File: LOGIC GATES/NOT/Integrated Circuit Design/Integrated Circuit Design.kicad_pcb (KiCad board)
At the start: 2 copper layers, 25 x 40 mm, 9 parts, among them J2 Conn_01x03_Socket, J3 Conn_01x03_Socket, Q1 QM6006D, Q3 QM6006D, U1 4011

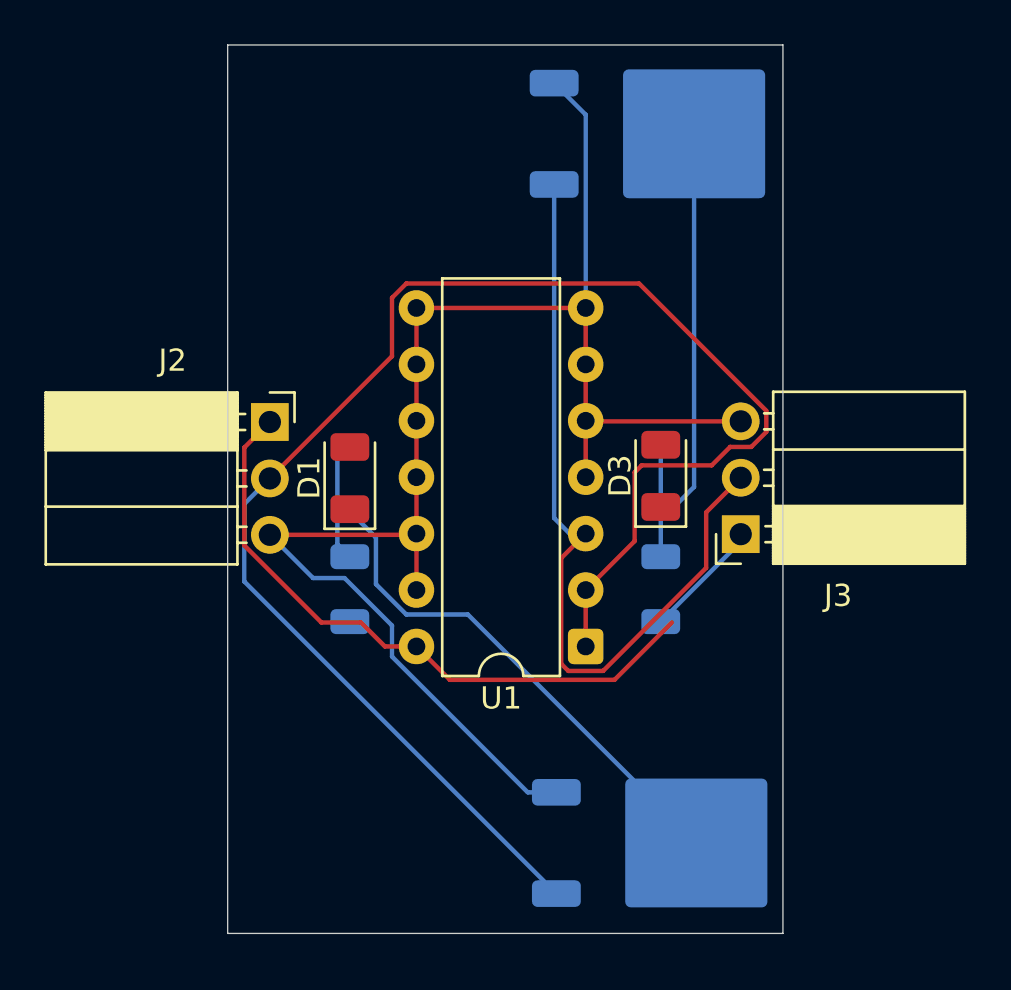
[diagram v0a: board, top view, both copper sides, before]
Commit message: Auto-update: 22.12.2025 16:16:21,18
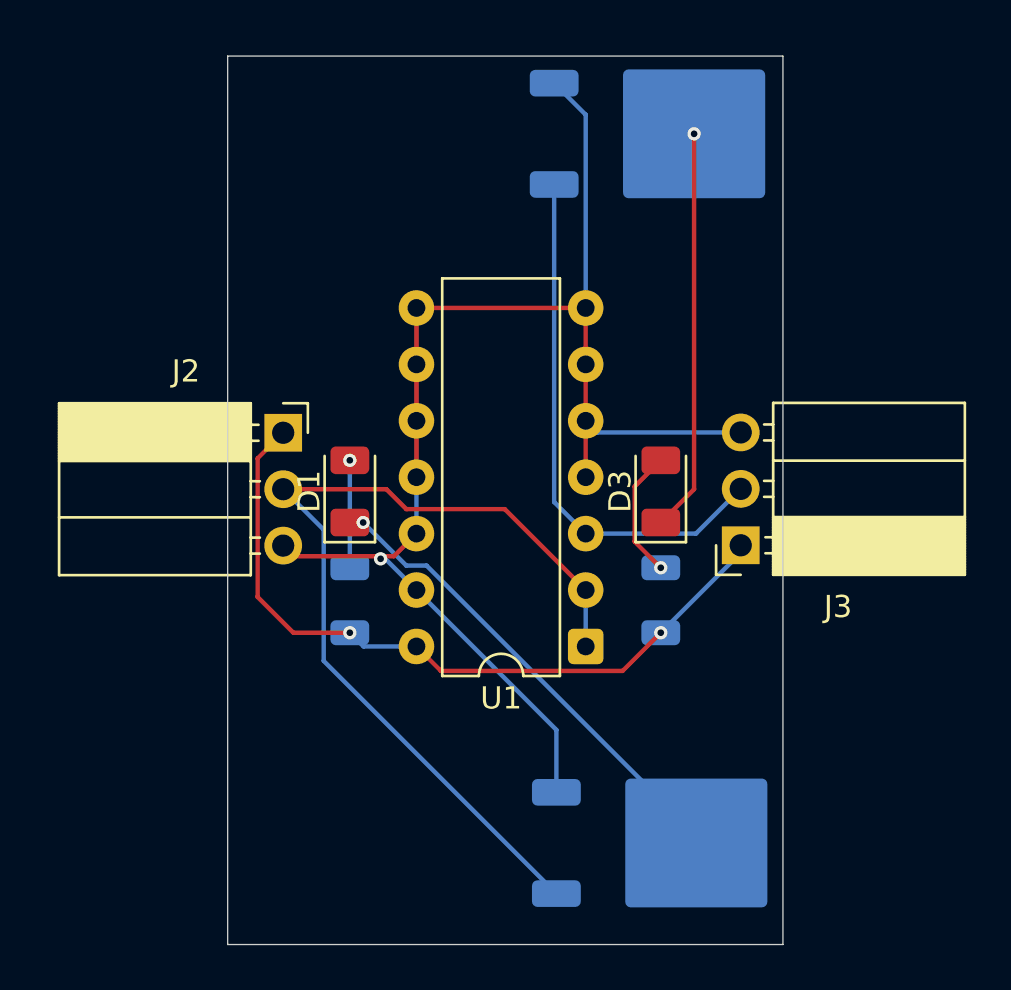
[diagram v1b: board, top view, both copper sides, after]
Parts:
- moved J2 0.77 mm to (92.5, 87.0)
- moved D3 0.70 mm to (109.5, 89.6)
- moved D1 0.60 mm to (95.5, 89.6)
- moved J3 0.50 mm to (113.1, 92.0)
- moved R1 0.50 mm to (95.5, 94.5)
- moved R3 0.50 mm to (109.5, 94.5)
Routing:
- net Net-(J2-Pin_2): track 71.3 -> 41.3 mm
- net Net-(J3-Pin_2): track 36.3 -> 24.1 mm
- net Net-(J2-Pin_3): track 70.8 -> 63.8 mm, vias 0 -> 1
- net Net-(D1-K): track 23.0 -> 21.2 mm, vias 0 -> 1
- net Net-(D3-A): track 5.04 -> 5.81 mm, vias 0 -> 1
- net Net-(J2-Pin_1): track 34.3 -> 33.5 mm, vias 0 -> 2
- net Net-(D3-K): track 17.5 -> 18.1 mm, vias 0 -> 1
- net Net-(D1-A): track 5.50 -> 4.84 mm, vias 0 -> 1
